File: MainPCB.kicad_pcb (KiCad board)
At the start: 4 copper layers, 105 x 62.4 mm, 42 parts, among them J1 RaspberryPi, J10 Conn_01x02, J12 Conn_01x07, J2 Conn_01x03, J3 Screw_Terminal_01x02, J4 Conn_01x02, J5 Conn_01x06, J6 Conn_01x03_Pin, J8 Conn_01x12, J9 Conn_01x04, M1 Motor_DC, M2 Motor_DC, M3 Motor_DC, M4 Motor_DC, SW1 SW_SPDT, SW2 SW_SPDT, SW3 SW_SPDT, SW4 SW_SPDT, U1 Teensy4.1, U10 Compass, U11 V_Regulator5v, U12 RockerSwitch, U13 V_Regulator3.3v, U2 VNH Driver, U3 VNH Driver, U4 VNH Driver, U5 VNH Driver, U6 TSOP25xx

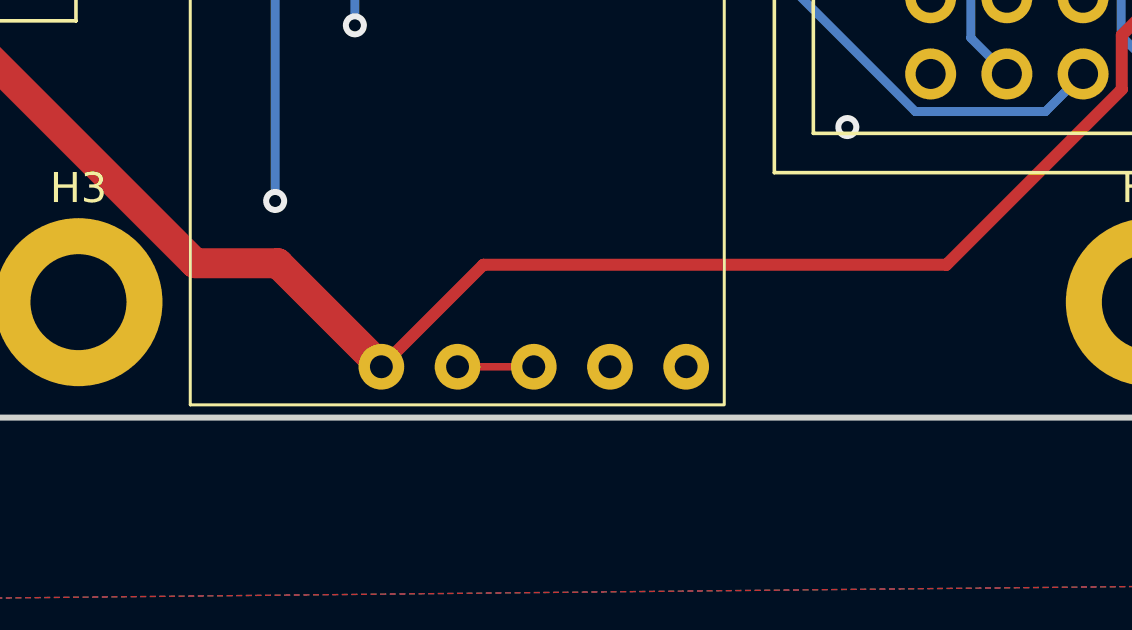
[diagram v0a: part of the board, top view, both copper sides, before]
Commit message: Fixed Regulator Pins
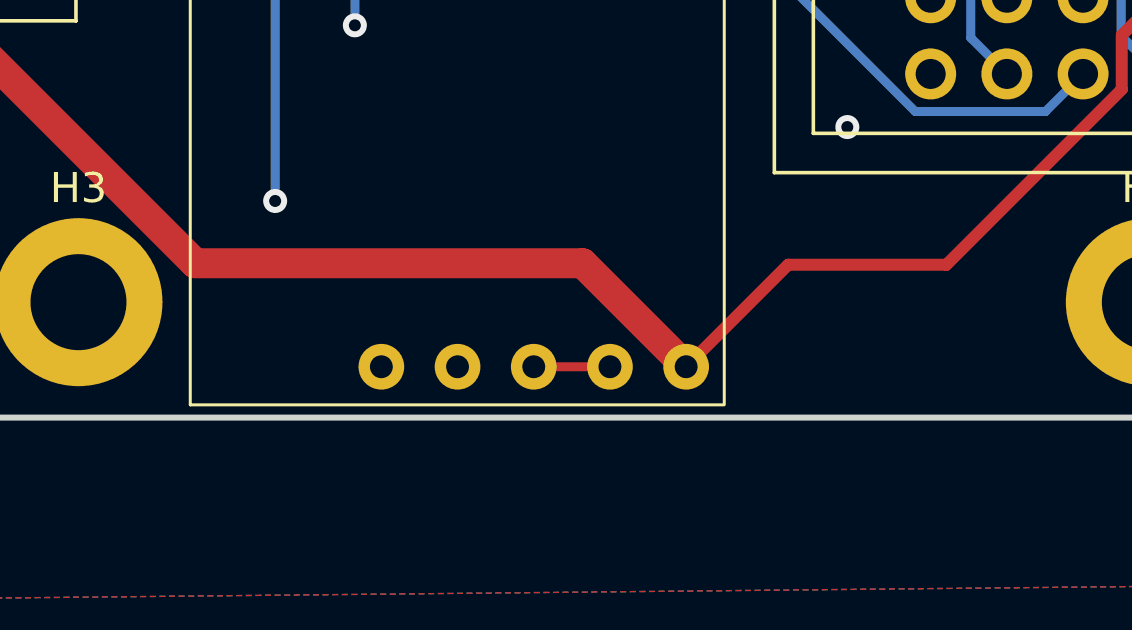
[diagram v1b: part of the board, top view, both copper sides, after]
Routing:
- net GND: track 398.8 -> 401.2 mm
- net 12V: track 240.5 -> 242.6 mm
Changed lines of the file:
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@@
 			)
 		)
+		(property ki_fp_filters "Connector*:*_1x??_*")
+		(sheetname "Root")
+		(sheetfile "MainPCB.kicad_sch")
 		(attr through_hole)
 		(fp_line
@@
 			(remove_unused_layers no)
 			(net 1 "GND")
-			(pinfunction "IN-")
+			(pinfunction "OUT-")
 			(pintype "input")
 		)
@@
 			)
 		)
+		(property ki_fp_filters "Connector*:*_1x??_*")
+		(sheetname "Root")
+		(sheetfile "MainPCB.kicad_sch")
 		(attr through_hole)
 		(fp_line
@@
 			)
 		)
-		(sheetname "Root")
-		(sheetfile "MainPCB.kicad_sch")
 		(attr through_hole)
 		(fp_rect
@@
 		)
 		(pad "1" thru_hole circle
-			(at 16.53 -1.27)
+			(at 6.37 -1.27)
 			(size 1.524 1.524)
 			(drill 0.762)
 			(layers "*.Cu" "*.Mask")
 			(remove_unused_layers no)
+			(pinfunction "OUT+")
+			(pintype "input")
 		)
 		(pad "3" thru_hole circle
-			(at 13.99 -1.27)
+			(at 8.91 -1.27)
 			(size 1.524 1.524)
 			(drill 0.762)
@@
 		)
 		(pad "4" thru_hole circle
-			(at 8.91 -1.27)
+			(at 11.45 -1.27)
 			(size 1.524 1.524)
 			(drill 0.762)
@@
 			(remove_unused_layers no)
 			(net 1 "GND")
-			(pinfunction "OUT-")
+			(pinfunction "IN-")
 			(pintype "input")
 		)
 		(pad "4" thru_hole circle
-			(at 11.45 -1.27)
+			(at 13.99 -1.27)
 			(size 1.524 1.524)
 			(drill 0.762)
@@
 			(remove_unused_layers no)
 			(net 1 "GND")
-			(pinfunction "OUT-")
+			(pinfunction "IN-")
 			(pintype "input")
 		)
 		(pad "5" thru_hole circle
-			(at 6.37 -1.27)
+			(at 16.53 -1.27)
 			(size 1.524 1.524)
 			(drill 0.762)
@@
 	)
 	(segment
-		(start 135.01 123.96)
-		(end 137.55 123.96)
-		(width 0.25)
+		(start 125.12 86.2)
+		(end 130.72 80.6)
+		(width 0.3)
 		(layer "F.Cu")
 		(net 1)
 	)
 	(segment
-		(start 125.12 86.2)
-		(end 130.72 80.6)
+		(start 137.55 123.96)
+		(end 140.09 123.96)
 		(width 0.3)
 		(layer "F.Cu")
@@
 	)
 	(segment
+		(start 120.6927 125.1439)
+		(end 113.9324 118.3836)
+		(width 0.3)
+		(layer "In1.Cu")
+		(net 1)
+	)
+	(segment
 		(start 177.8 120.2181)
 		(end 177.8 117.6)
@@
 	)
 	(segment
+		(start 136.3661 125.1439)
+		(end 120.6927 125.1439)
+		(width 0.3)
+		(layer "In1.Cu")
+		(net 1)
+	)
+	(segment
 		(start 162.8 81.3)
 		(end 166.9 85.4)
@@
 	)
 	(segment
+		(start 137.55 123.96)
+		(end 136.3661 125.1439)
+		(width 0.3)
+		(layer "In1.Cu")
+		(net 1)
+	)
+	(segment
 		(start 150.4261 97.0839)
 		(end 150.4261 111.3061)
@@
 	)
 	(segment
-		(start 134.0061 125.1439)
-		(end 120.6927 125.1439)
-		(width 0.3)
-		(layer "In1.Cu")
-		(net 1)
-	)
-	(segment
 		(start 137.578 79.3992)
 		(end 137.578 71.4128)
@@
 	)
 	(segment
-		(start 135.12 124.03)
-		(end 134.0061 125.1439)
-		(width 0.3)
-		(layer "In1.Cu")
-		(net 1)
-	)
-	(segment
 		(start 174.82 123.1981)
 		(end 177.8 120.2181)
@@
 	)
 	(segment
-		(start 120.6927 125.1439)
-		(end 113.9324 118.3836)
-		(width 0.3)
-		(layer "In1.Cu")
-		(net 1)
-	)
-	(segment
 		(start 113.27 111.2451)
 		(end 114.92 112.8951)
@@
 	)
 	(segment
-		(start 114.887968 109.14)
-		(end 114.54 109.14)
-		(width 1)
+		(start 146.03 120.56)
+		(end 151.307767 120.56)
+		(width 0.4)
 		(layer "F.Cu")
 		(net 3)
@@
 	)
 	(segment
-		(start 132.47 123.96)
-		(end 135.87 120.56)
-		(width 0.4)
+		(start 142.63 123.96)
+		(end 139.18 120.51)
+		(width 1)
 		(layer "F.Cu")
 		(net 3)
 	)
 	(segment
-		(start 157.15 112.91)
-		(end 158.4 111.66)
+		(start 157.15 114.717767)
+		(end 157.15 112.91)
 		(width 0.4)
 		(layer "F.Cu")
@@
 	)
 	(segment
-		(start 132.47 123.96)
-		(end 129.02 120.51)
+		(start 126.257968 120.51)
+		(end 114.887968 109.14)
+		(width 1)
+		(layer "F.Cu")
+		(net 3)
+	)
+	(segment
+		(start 114.887968 109.14)
+		(end 114.54 109.14)
 		(width 1)
 		(layer "F.Cu")
@@
 	)
 	(segment
-		(start 135.87 120.56)
-		(end 151.307767 120.56)
+		(start 157.15 112.91)
+		(end 158.4 111.66)
 		(width 0.4)
 		(layer "F.Cu")
@@
 	)
 	(segment
-		(start 157.15 114.717767)
-		(end 157.15 112.91)
+		(start 151.307767 120.56)
+		(end 157.15 114.717767)
 		(width 0.4)
 		(layer "F.Cu")
@@
 	)
 	(segment
-		(start 151.307767 120.56)
-		(end 157.15 114.717767)
+		(start 142.63 123.96)
+		(end 146.03 120.56)
 		(width 0.4)
 		(layer "F.Cu")
@@
 	)
 	(segment
-		(start 129.02 120.51)
+		(start 139.18 120.51)
 		(end 126.257968 120.51)
 		(width 1)
@@
 	)
 	(segment
-		(start 126.257968 120.51)
-		(end 114.887968 109.14)
-		(width 1)
-		(layer "F.Cu")
-		(net 3)
-	)
-	(segment
 		(start 89.56 86.2)
 		(end 95.84 92.48)
@@
 	)
 	(segment
-		(start 171.6592 109.5092)
-		(end 146.8384 109.5092)
+		(start 175.3 116.7303)
+		(end 174.05 115.4803)
 		(width 2)
 		(layer "In2.Cu")
@@
 	)
 	(segment
-		(start 146.8384 109.5092)
-		(end 140.09 116.2576)
+		(start 135.01 121.3376)
+		(end 135.01 123.96)
 		(width 2)
 		(layer "In2.Cu")
@@
 	)
 	(segment
-		(start 174.05 111.9)
-		(end 171.6592 109.5092)
+		(start 174.05 115.4803)
+		(end 174.05 111.9)
 		(width 2)
 		(layer "In2.Cu")
@@
 	)
 	(segment
-		(start 175.3 116.7303)
-		(end 174.05 115.4803)
+		(start 171.6592 109.5092)
+		(end 146.8384 109.5092)
 		(width 2)
 		(layer "In2.Cu")
@@
 	)
 	(segment
-		(start 175.3 117.6)
-		(end 175.3 116.7303)
+		(start 146.8384 109.5092)
+		(end 135.01 121.3376)
 		(width 2)
 		(layer "In2.Cu")
@@
 	)
 	(segment
-		(start 174.05 115.4803)
-		(end 174.05 111.9)
+		(start 175.3 117.6)
+		(end 175.3 116.7303)
 		(width 2)
 		(layer "In2.Cu")
@@
 	)
 	(segment
-		(start 140.09 116.2576)
-		(end 140.09 123.96)
+		(start 174.05 111.9)
+		(end 171.6592 109.5092)
 		(width 2)
 		(layer "In2.Cu")
